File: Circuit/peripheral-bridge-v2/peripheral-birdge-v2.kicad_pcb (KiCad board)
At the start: 2 copper layers, 50 x 54.3 mm, 74 parts, among them CON1 Conn-Edge-PCIE-x1, J1 To DVL, J2 Pressure Sensor, J3 Solenoid, J4 USB_OTG, P1 Solenoid Power, Q1 BSS138, U1 FT2232H, U2 93LC56BT-I/OT, U3 ADM3251E, U4 ADC101S021, U5 ACPL-247-500E, U6 ACPL-247-500E, U7 LM1117-33, Y1 12MHz

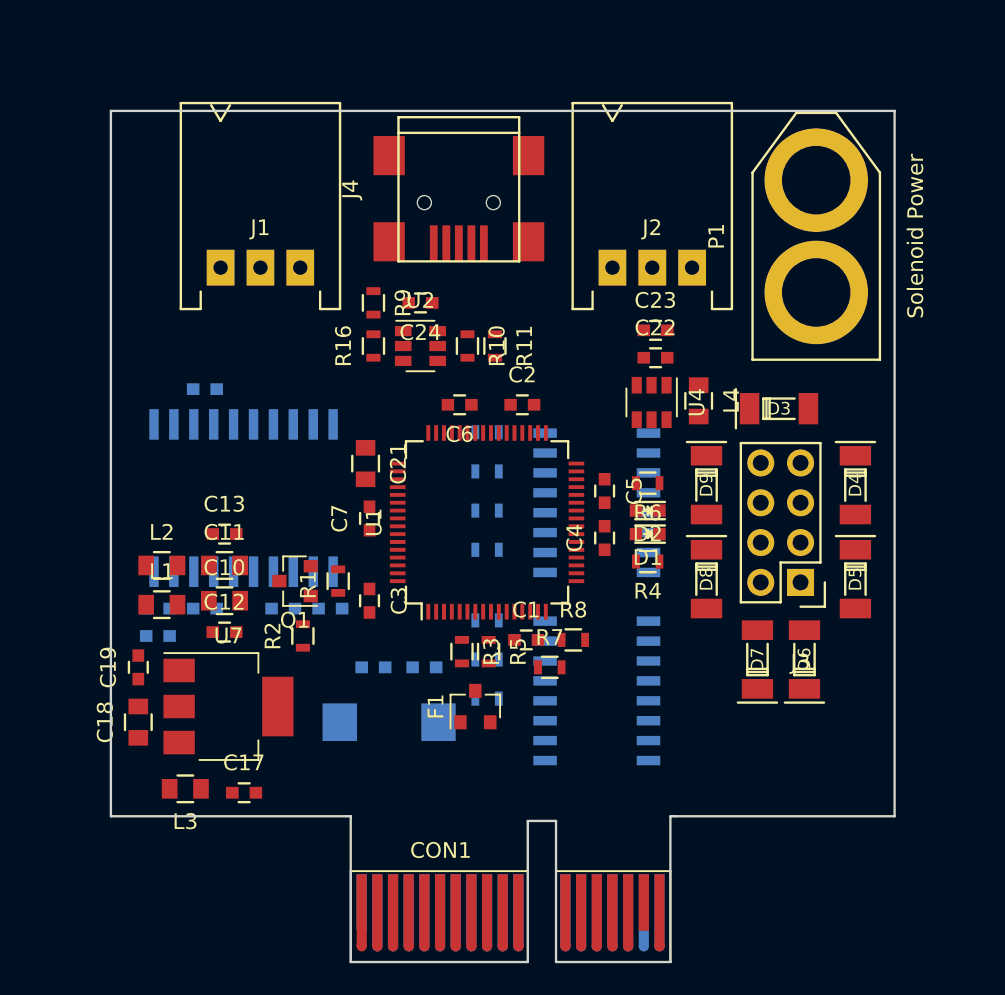
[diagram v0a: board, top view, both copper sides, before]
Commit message: Finished PCB Routing
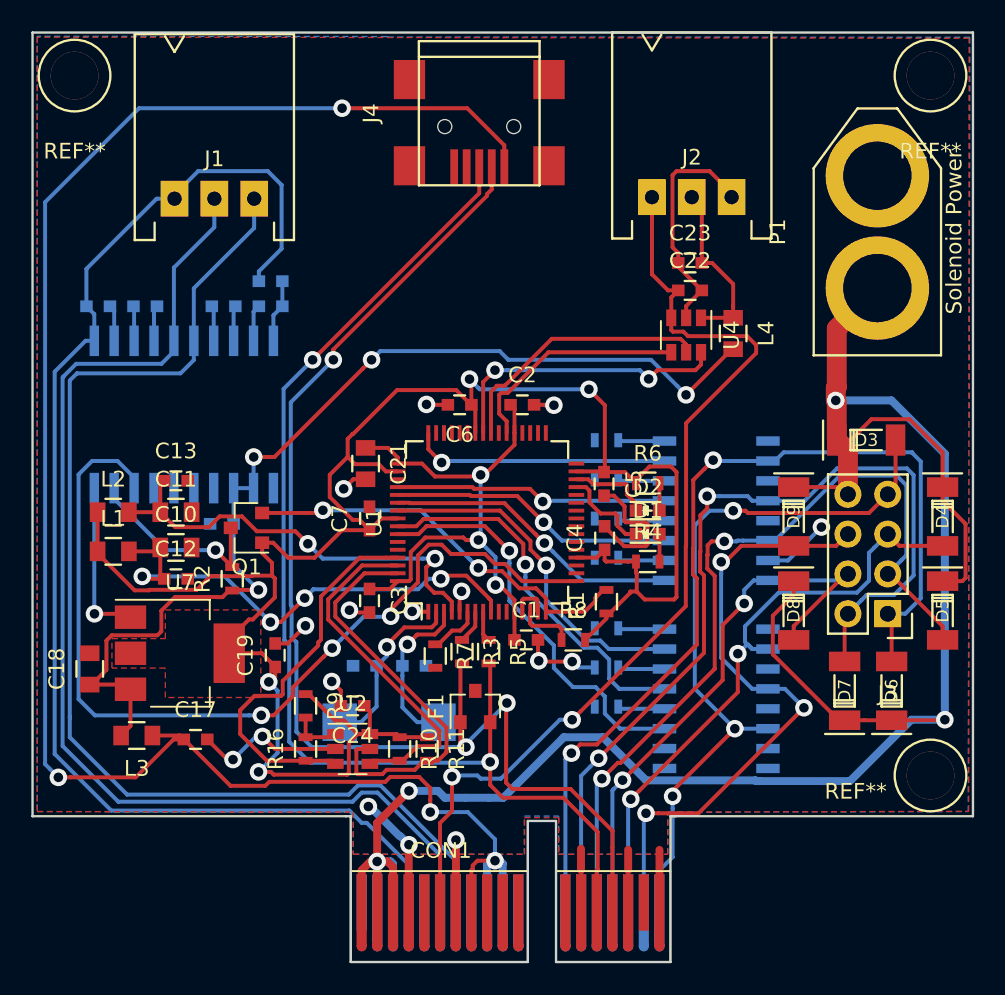
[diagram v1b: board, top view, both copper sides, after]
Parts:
- added REF**: 1pin, Connectors:1pin, F.Cu at (177.3, 117.4)
- added REF**: 1pin, Connectors:1pin, F.Cu at (177.3, 72.7)
- added REF**: 1pin, Connectors:1pin, F.Cu at (122.7, 72.7)
- moved C24 26.1 mm to (140.4, 113.0)
- moved R10 26.1 mm to (143.4, 115.7)
- moved R11 26.1 mm to (145.2, 115.7)
- moved R16 26.1 mm to (137.4, 115.7)
- moved R9 26.1 mm to (137.4, 113.0)
- moved U2 26.1 mm to (140.4, 115.7)
- moved C20 24.3 mm to (124.2, 87.5), turned to 0 degrees
- moved C9 23.7 mm to (135.2, 85.9), turned to 180 degrees
- moved C16 21.2 mm to (127.2, 87.5), turned to 0 degrees
- moved C8 20.6 mm to (135.2, 87.5), turned to 180 degrees
- moved C15 19.3 mm to (132.2, 87.5), turned to 180 degrees
- moved R1 17.2 mm to (156.6, 106.3)
- moved C19 8.77 mm to (135.5, 109.7)
- moved C14 8.66 mm to (132.1, 101.3), turned to 180 degrees
- moved R12 7.64 mm to (156.6, 96.0)
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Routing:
- net +12V: track 0.00 -> 142.2 mm, vias 0 -> 4
- net +3V3: track 0.00 -> 132.4 mm, vias 0 -> 4
- net +5Vin: track 0.00 -> 119.2 mm, vias 0 -> 4
- net 232_GND: track 0.00 -> 83.2 mm
- net D-: track 0.00 -> 80.9 mm, vias 0 -> 3
- net GND: track 0.00 -> 76.9 mm, vias 0 -> 17
- net D+: track 0.00 -> 76.3 mm, vias 0 -> 2
- net Tx: track 0.00 -> 74.7 mm
- net Rx: track 0.00 -> 73.1 mm
- net VBUS: track 0.00 -> 67.2 mm, vias 0 -> 4
- net Analog_In: track 0.00 -> 62.5 mm, vias 0 -> 2
- net Sol1: track 0.00 -> 61.6 mm, vias 0 -> 2
- net Sol2: track 0.00 -> 59.5 mm, vias 0 -> 2
- net Net-(U1-Pad17): track 0.00 -> 59.0 mm, vias 0 -> 3
- net Sol3: track 0.00 -> 53.4 mm, vias 0 -> 2
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- added copper zone on F.Cu, net +3V3
- added copper zone on B.Cu, net GND
- added copper zone on F.Cu, net GND
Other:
- board size 50 x 54.3 mm -> 60 x 59.3 mm
- net class Default: clearance 0.2 -> 0.2032; trace_width 0.25 -> 0.254; via_dia 0.6 -> 1.1176; via_drill 0.4 -> 0.6096
- rule trace_clearance: 0.2 -> 0.2032
- rule trace_min: 0.2 -> 0.254
- rule via_min_drill: 0.3 -> 0.2
- rule via_min_size: 0.4 -> 1.016
